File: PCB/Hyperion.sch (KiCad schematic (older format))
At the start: 118 parts, among them SW1 SW_PUSH, SW10 SW_PUSH, SW11 SW_PUSH, SW12 SW_PUSH, SW13 SW_PUSH, SW14 SW_PUSH, SW15 SW_PUSH, SW16 SW_PUSH, SW17 SW_PUSH, SW18 SW_PUSH, SW19 SW_PUSH, SW2 SW_PUSH, SW20 SW_PUSH, SW21 SW_PUSH, SW22 SW_PUSH, SW23 SW_PUSH, SW24 SW_PUSH, SW25 SW_PUSH, SW26 SW_PUSH, SW27 SW_PUSH, SW28 SW_PUSH, SW29 SW_PUSH, SW3 SW_PUSH, SW30 SW_PUSH, SW31 SW_PUSH, SW32 SW_PUSH, SW33 SW_PUSH, SW34 SW_PUSH, SW35 SW_PUSH, SW36 SW_PUSH, SW37 SW_PUSH, SW38 SW_PUSH, SW39 SW_PUSH, SW4 SW_PUSH, SW40 SW_PUSH, SW41 SW_PUSH, SW42 SW_PUSH, SW43 SW_PUSH, SW44 SW_PUSH, SW45 SW_PUSH, SW46 SW_PUSH, SW47 SW_PUSH, SW48 SW_PUSH, SW49 SW_PUSH, SW5 SW_PUSH, SW50 SW_PUSH, SW51 SW_PUSH, SW52 SW_PUSH, SW53 SW_PUSH, SW54 SW_PUSH, SW55 SW_PUSH, SW56 SW_PUSH, SW57 SW_PUSH, SW58 SW_PUSH, SW59 SW_PUSH, SW6 SW_PUSH, SW7 SW_PUSH, SW8 SW_PUSH, SW9 SW_PUSH, U1 ProMicro

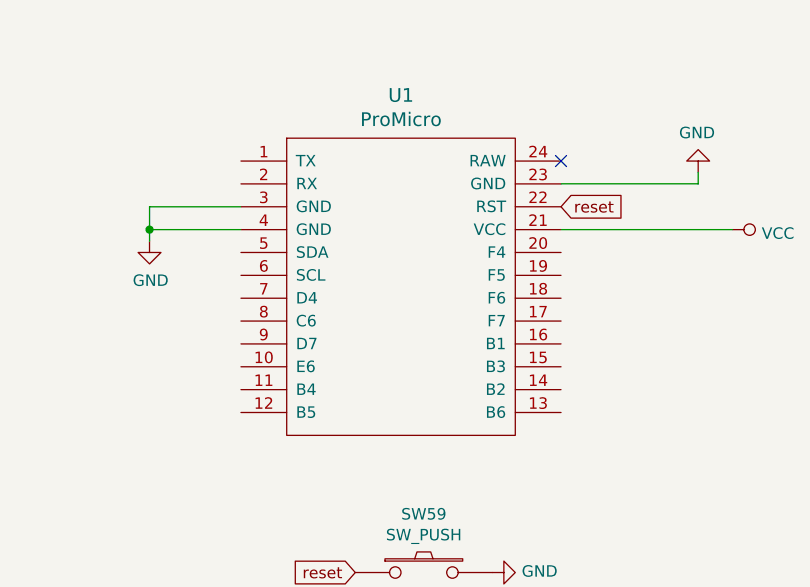
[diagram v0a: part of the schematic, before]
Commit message: pcb first draft
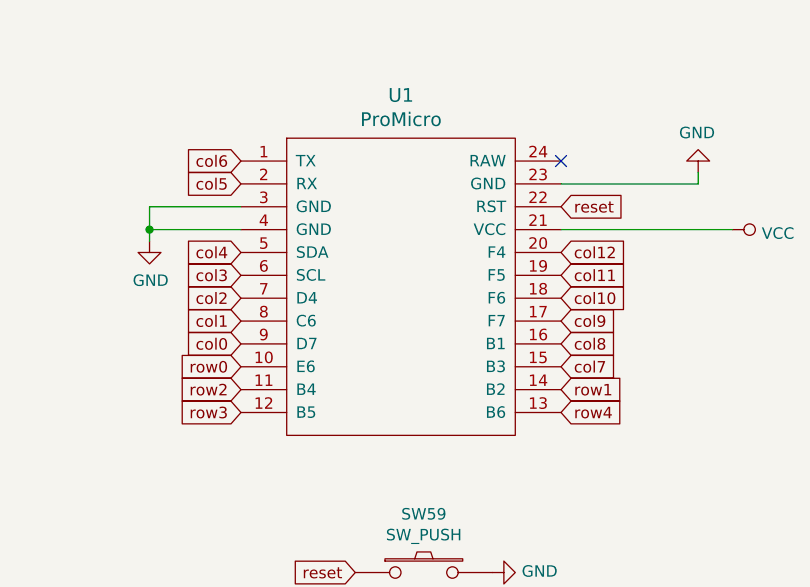
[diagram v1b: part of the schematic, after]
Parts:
- D1, D10, D11, D12, D13, D14, D15, D16, D17, D18, D19, D2, D20, D21, D22, D23, D24, D25, D26, D27, D28, D29, D3, D30, D31, D32, D33, D34, D35, D36, D37, D38, D39, D4, D40, D41, D42, D43, D44, D45, D46, D47, D48, D49, D5, D50, D51, D52, D53, D54, D55, D56, D57, D58, D6, D7, D8, D9: footprint Diode_THT:D_DO-35_SOD27_P7.62mm_Horizontal -> Diode_SMD:D_SOD-123
- SW1, SW10, SW11, SW12, SW13, SW14, SW15, SW16, SW17, SW18, SW19, SW2, SW20, SW21, SW22, SW23, SW24, SW25, SW26, SW27, SW28, SW29, SW3, SW30, SW31, SW32, SW33, SW34, SW35, SW36, SW37, SW38, SW39, SW4, SW40, SW41, SW42, SW43, SW44, SW45, SW46, SW47, SW48, SW49, SW5, SW50, SW51, SW52, SW53, SW54, SW55, SW56, SW57, SW58, SW6, SW7, SW8, SW9: footprint (none) -> emptystring:CherryMX_Hotswap_Back
- SW59: footprint (none) -> kbd:ResetSW
- U1: footprint (none) -> emptystring:ProMicro_v2_Backside
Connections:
- net col0: now also U1.9 (D7)
- net col1: now also U1.8 (C6)
- net col10: now also U1.18 (F6)
- net col11: now also U1.19 (F5)
- net col12: now also U1.20 (F4)
- net col2: now also U1.7 (D4)
- net col3: now also U1.6 (SCL)
- net col4: now also U1.5 (SDA)
- net col5: now also U1.2 (RX)
- net col6: now also U1.1 (TX)
- net col7: now also U1.15 (B3)
- net col8: now also U1.16 (B1)
- net col9: now also U1.17 (F7)
- net row0: now also U1.10 (E6)
- net row1: now also U1.14 (B2)
- net row2: now also U1.11 (B4)
- net row3: now also U1.12 (B5)
- net row4: now also U1.13 (B6)
